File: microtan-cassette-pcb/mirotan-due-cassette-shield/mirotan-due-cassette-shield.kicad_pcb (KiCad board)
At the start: 2 copper layers, 20 parts, among them J1 Conn_01x03, J2 Conn_01x04, Q1 BC547, Q2 BC547, SW1 SW_SPST, SW2 SW_SPST, SW3 SW_SPST

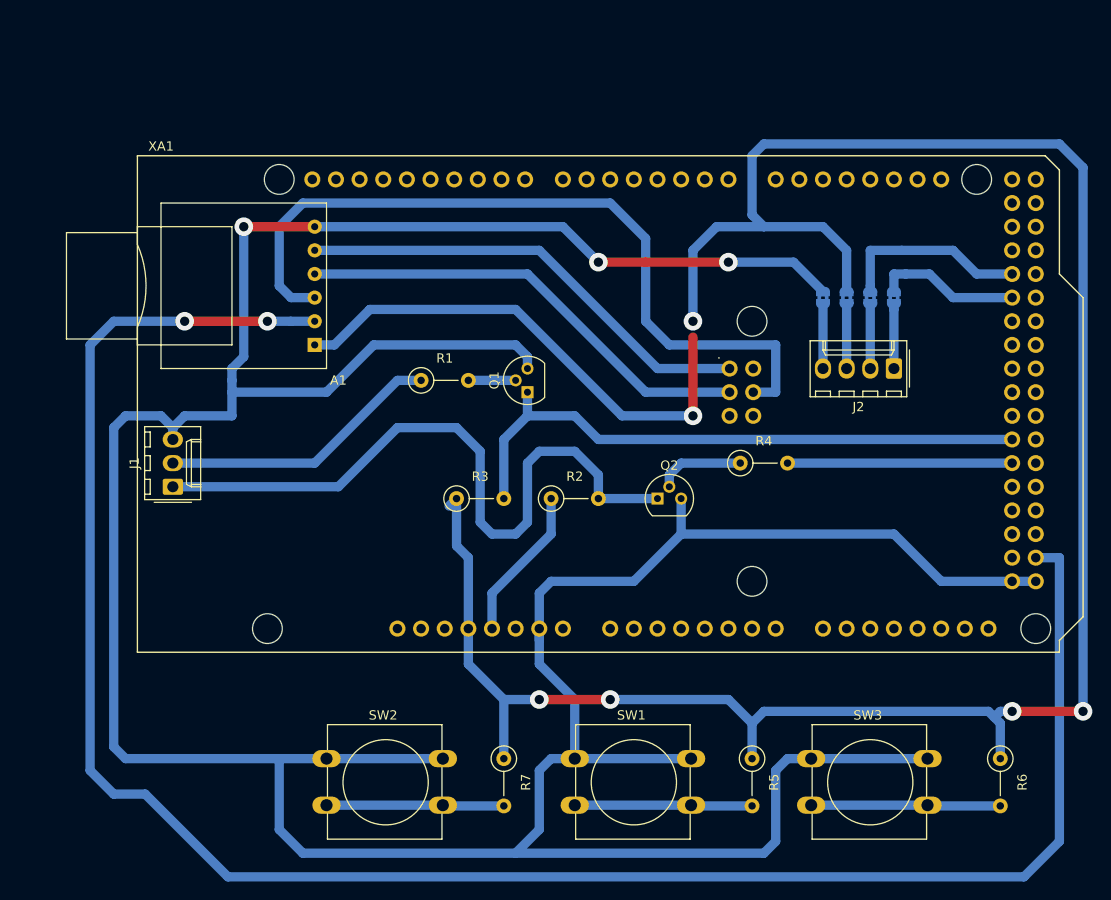
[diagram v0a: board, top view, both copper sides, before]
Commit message: First fab files.
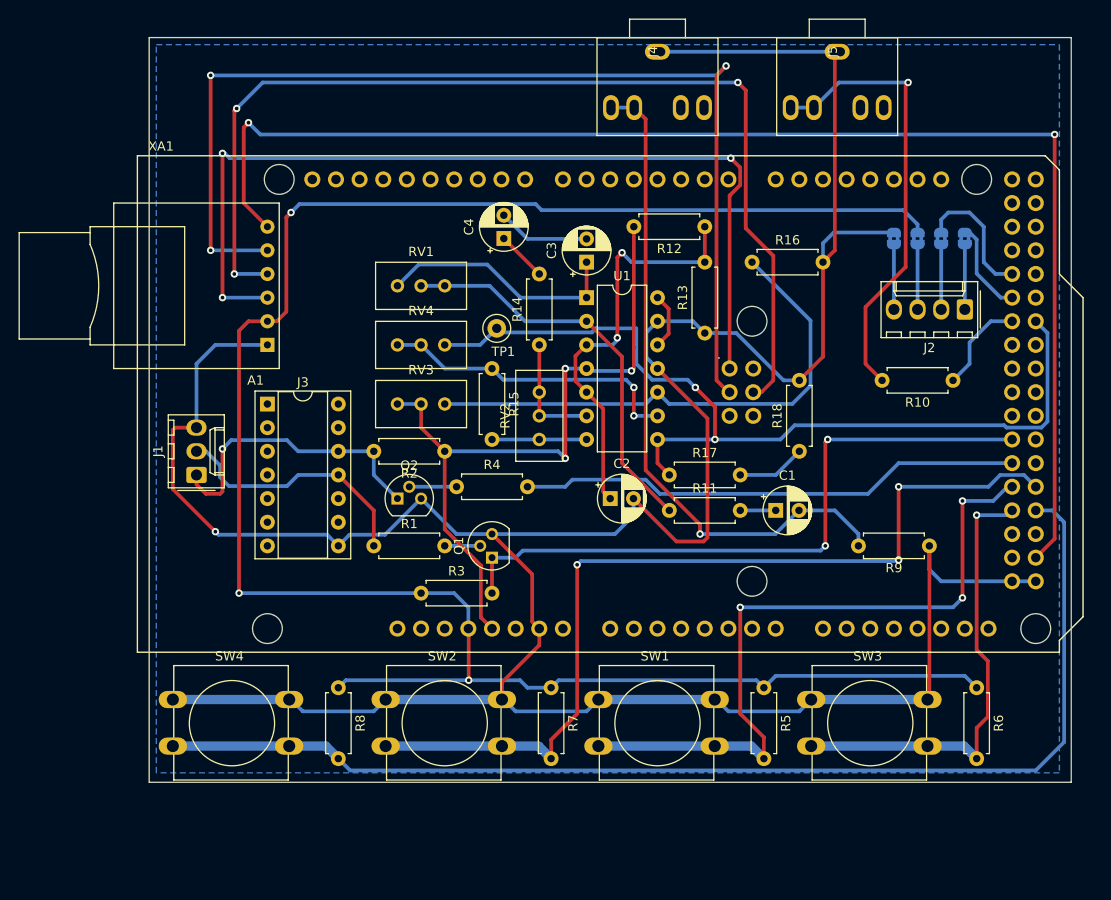
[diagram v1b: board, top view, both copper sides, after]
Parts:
- added C1: 10uF, Capacitor_THT:CP_Radial_D5.0mm_P2.50mm, F.Cu at (68.6, -19.1)
- added C2: 10uF, Capacitor_THT:CP_Radial_D5.0mm_P2.50mm, F.Cu at (50.8, -20.3)
- added C3: 10uF, Capacitor_THT:CP_Radial_D5.0mm_P2.50mm, F.Cu at (48.3, -45.7)
- added C4: 10uF, Capacitor_THT:CP_Radial_D5.0mm_P2.50mm, F.Cu at (39.4, -48.3)
- added J3: Conn_02x07_Counter_Clockwise, Package_DIP:DIP-14_W7.62mm_Socket, F.Cu at (14.0, -30.5)
- added J4: Barrel_Jack_Switch-truconnect-20-0138, mirotan-due-cassette-shield:truconnect-20-0138-mono-socket, F.Cu at (55.9, -68.3)
- added J5: Barrel_Jack_Switch-truconnect-20-0138, mirotan-due-cassette-shield:truconnect-20-0138-mono-socket, F.Cu at (75.2, -68.3)
- added R10: 1k, Resistor_THT:R_Axial_DIN0207_L6.3mm_D2.5mm_P7.62mm_Horizontal, F.Cu at (87.6, -33.0)
- added R11: 10k, Resistor_THT:R_Axial_DIN0207_L6.3mm_D2.5mm_P7.62mm_Horizontal, F.Cu at (57.1, -19.1)
- added R12: 100k, Resistor_THT:R_Axial_DIN0207_L6.3mm_D2.5mm_P7.62mm_Horizontal, F.Cu at (61.0, -49.5)
- added R13: 100k, Resistor_THT:R_Axial_DIN0207_L6.3mm_D2.5mm_P7.62mm_Horizontal, F.Cu at (61.0, -38.1)
- added R14: 2k2, Resistor_THT:R_Axial_DIN0207_L6.3mm_D2.5mm_P7.62mm_Horizontal, F.Cu at (43.2, -36.8)
- added R15: 2k2, Resistor_THT:R_Axial_DIN0207_L6.3mm_D2.5mm_P7.62mm_Horizontal, F.Cu at (38.1, -34.3)
- added R16: 100k, Resistor_THT:R_Axial_DIN0207_L6.3mm_D2.5mm_P7.62mm_Horizontal, F.Cu at (66.0, -45.7)
- added R17: 2k2, Resistor_THT:R_Axial_DIN0207_L6.3mm_D2.5mm_P7.62mm_Horizontal, F.Cu at (57.1, -22.9)
- added R18: 2k2, Resistor_THT:R_Axial_DIN0207_L6.3mm_D2.5mm_P7.62mm_Horizontal, F.Cu at (71.1, -25.4)
- added R8: 1k, Resistor_THT:R_Axial_DIN0207_L6.3mm_D2.5mm_P7.62mm_Horizontal, F.Cu at (21.6, 0.00)
- added R9: 100k, Resistor_THT:R_Axial_DIN0207_L6.3mm_D2.5mm_P7.62mm_Horizontal, F.Cu at (85.1, -15.2)
- added RV1: 200k, Potentiometer_THT:Potentiometer_Bourns_3296W_Vertical, F.Cu at (33.0, -43.2)
- added RV2: 500k, Potentiometer_THT:Potentiometer_Bourns_3296W_Vertical, F.Cu at (43.2, -31.8)
- added RV3: 200k, Potentiometer_THT:Potentiometer_Bourns_3296W_Vertical, F.Cu at (33.0, -30.5)
- added RV4: 500k, Potentiometer_THT:Potentiometer_Bourns_3296W_Vertical, F.Cu at (33.0, -36.8)
- added SW4: SW_SPST, Button_Switch_THT:SW_PUSH-12mm, F.Cu at (3.81, 1.27)
- added TP1: TestPoint, TestPoint:TestPoint_Loop_D1.80mm_Drill1.0mm_Beaded, F.Cu at (38.6, -38.6)
- added U1: LM324, Package_DIP:DIP-14_W7.62mm, F.Cu at (48.3, -41.9)
- A1: value SD_Card_Module -> SD_Card_Module_catalex
- R1, R2, R3, R4, R5, R6, R7: footprint Resistor_THT:R_Axial_DIN0207_L6.3mm_D2.5mm_P5.08mm_Vertical -> Resistor_THT:R_Axial_DIN0207_L6.3mm_D2.5mm_P7.62mm_Horizontal
- moved R4 30.6 mm to (34.3, -21.6)
- moved Q2 27.9 mm to (27.9, -20.3)
- moved R1 18.5 mm to (25.4, -15.2)
- moved Q1 18.2 mm to (38.1, -14.0)
- moved R2 12.5 mm to (33.0, -25.4), turned to 180 degrees
- moved R3 10.9 mm to (30.5, -10.2)
- moved J2 9.92 mm to (88.9, -40.6)
- moved JP1 9.92 mm to (88.9, -48.3)
- moved JP2 9.92 mm to (86.4, -48.3)
- moved JP4 9.92 mm to (81.3, -48.3)
- moved JP3 9.92 mm to (83.8, -48.3)
- moved R7 9.16 mm to (44.5, 0.00)
- moved SW2 8.98 mm to (26.7, 1.27)
- moved R6 8.03 mm to (90.2, 0.00)
- moved R5 7.73 mm to (67.3, 0.00)
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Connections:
- A1 pad 1: +3V3 -> GND
- A1 pad 2: Net-(A1-Pad2) -> +3V3
- A1 pad 6: GND -> Net-(A1-Pad6)
- XA1 pad D32: Net-(XA1-PadD32) -> CAS_OUT
- XA1 pad D33: Net-(XA1-PadD33) -> CAS_IN
- XA1 pad D46: Net-(XA1-PadD46) -> Net-(R5-Pad2)
- XA1 pad D47: Net-(XA1-PadD47) -> Net-(R7-Pad2)
- XA1 pad D48: Net-(XA1-PadD48) -> Net-(R6-Pad2)
- XA1 pad D53: Net-(A1-Pad2) -> Net-(A1-Pad6)
- XA1 pad MISO: Net-(A1-Pad5) -> Net-(A1-Pad3)
- XA1 pad MOSI: Net-(A1-Pad3) -> Net-(A1-Pad4)
- XA1 pad SCK: Net-(A1-Pad4) -> Net-(A1-Pad5)
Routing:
- net Net-(A1-Pad2): track 214.4 -> 0.00 mm, vias 2 -> 0
- net Net-(A1-Pad6): track 0.00 -> 145.9 mm, vias 0 -> 2
- net Net-(R8-Pad2): track 0.00 -> 125.3 mm
- net CAS_IN: track 0.00 -> 97.9 mm, vias 0 -> 2
- net Net-(R7-Pad2): track 19.1 -> 98.7 mm, vias 0 -> 3
- net +3V3: track 293.8 -> 218.5 mm, vias 6 -> 3
- net Net-(C1-Pad2): track 0.00 -> 71.6 mm, vias 0 -> 1
- net Net-(A1-Pad5): track 49.8 -> 116.8 mm, vias 0 -> 3
- net GND: track 403.6 -> 340.3 mm, vias 3 -> 1
- net Net-(A1-Pad4): track 49.8 -> 112.7 mm, vias 0 -> 3
- net +5V: track 16.6 -> 75.6 mm, vias 0 -> 3
- net Net-(R5-Pad2): track 19.1 -> 76.3 mm, vias 0 -> 3
- net Net-(R16-Pad1): track 0.00 -> 57.0 mm
- net Net-(J5-Pad4): track 0.00 -> 48.4 mm, vias 0 -> 1
- net Net-(C2-Pad1): track 0.00 -> 44.8 mm, vias 0 -> 2
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- added copper zone on B.Cu, net GND
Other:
- board outline added: 99.1 x 80 mm
